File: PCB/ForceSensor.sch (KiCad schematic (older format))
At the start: 4 parts

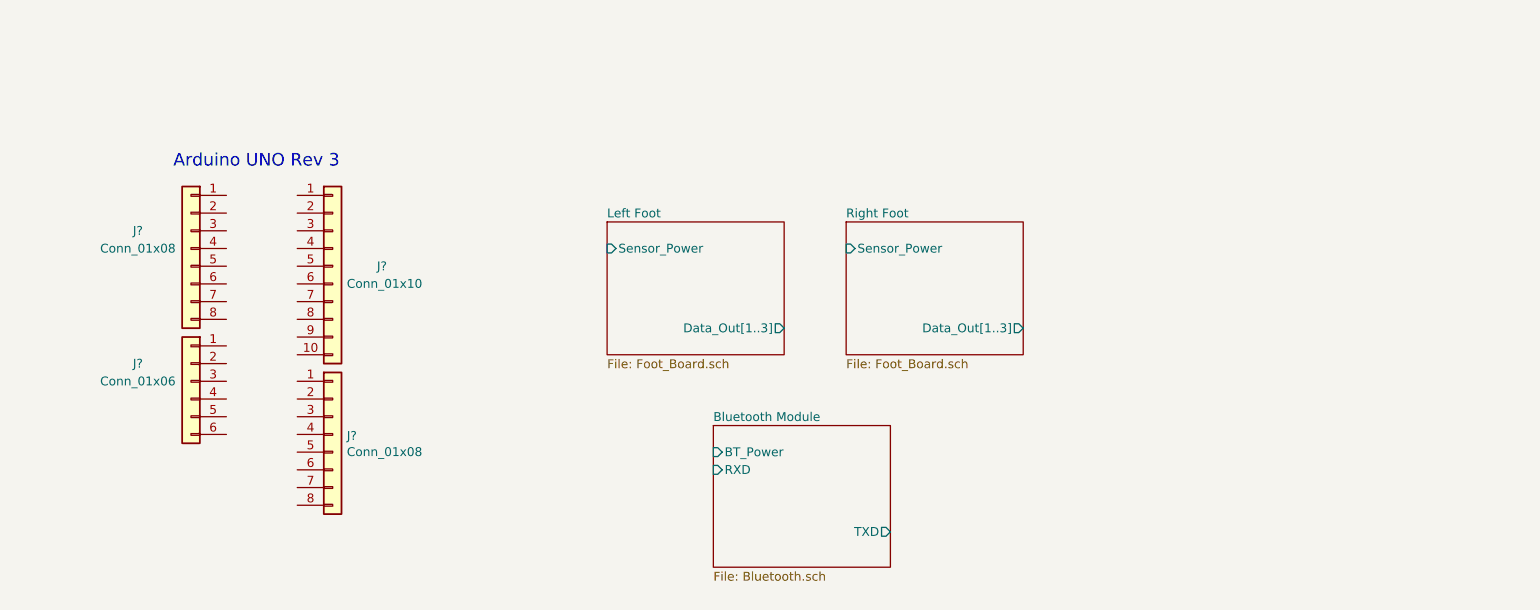
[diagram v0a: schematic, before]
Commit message: Finished schematic
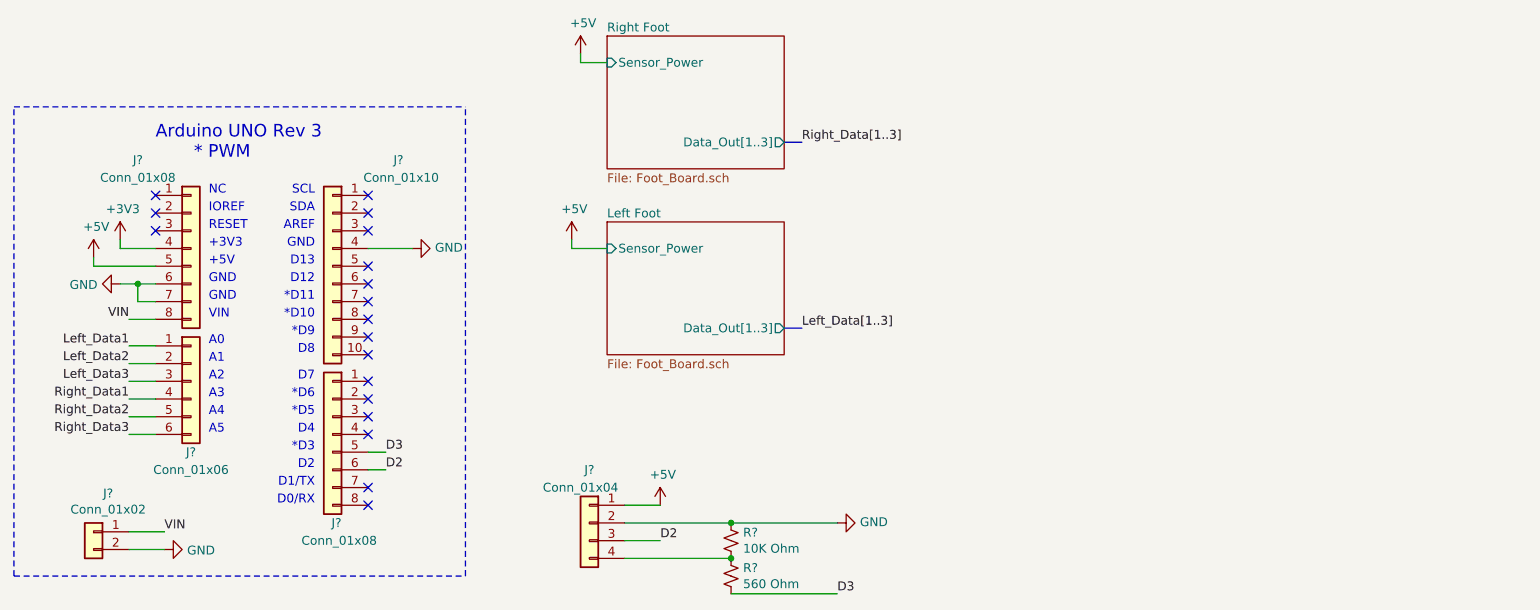
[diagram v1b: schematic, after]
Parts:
- added J?: Conn_01x04, symbol Connector_Generic:Conn_01x04
- added J?: Conn_01x02, symbol Connector_Generic:Conn_01x02
- added R?: 10K Ohm, symbol Device:R_Small_US
- added R?: 560 Ohm, symbol Device:R_Small_US
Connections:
- net GND: now reaches J?.4 (Pin_4)
- net GND: now also J?.6 (Pin_6), J?.7 (Pin_7), J?.2 (Pin_2), J?.2 (Pin_2), R?.1
- net D3: now reaches J?.5 (Pin_5)
- net D3: now also R?.2
- net D2: now reaches J?.6 (Pin_6)
- net D2: now also J?.3 (Pin_3)
- net +3V3: now reaches J?.4 (Pin_4)
- net +5V: now reaches J?.5 (Pin_5)
- net +5V: now also J?.1 (Pin_1)
- net VIN: now reaches J?.8 (Pin_8)
- net VIN: now also J?.1 (Pin_1)
- net Left_Data1: now reaches J?.1 (Pin_1)
- net Left_Data2: now reaches J?.2 (Pin_2)
- net Left_Data3: now reaches J?.3 (Pin_3)
- net Right_Data1: now reaches J?.4 (Pin_4)
- net Right_Data2: now reaches J?.5 (Pin_5)
- net Right_Data3: now reaches J?.6 (Pin_6)
- new net: J?.4 (Pin_4), R?.1, R?.2
- no-connect marks 0 -> 18
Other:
- note added: "*D10"
- note added: "*D11"
- note added: "*D3"
- note added: "*D5"
- note added: "*D6"
- note added: "*D9"
- note added: "+3V3"
- note added: "+5V"
- note added: "A0"
- note added: "A1"
- note added: "A2"
- note added: "A3"
- note added: "A4"
- note added: "A5"
- note added: "AREF"
- note added: "Arduino UNO Rev 3\n * PWM"
- note added: "D0/RX"
- note added: "D1/TX"
- note added: "D12"
- note added: "D13"
- note added: "D2"
- note added: "D4"
- note added: "D7"
- note added: "D8"
- note added: "GND"
- note added: "IOREF"
- note added: "NC"
- note added: "RESET"
- note added: "SCL"
- note added: "SDA"
- note added: "VIN"
- note removed: "Arduino UNO Rev 3"
- moved on the sheet: J?

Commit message: Small changes to schematic
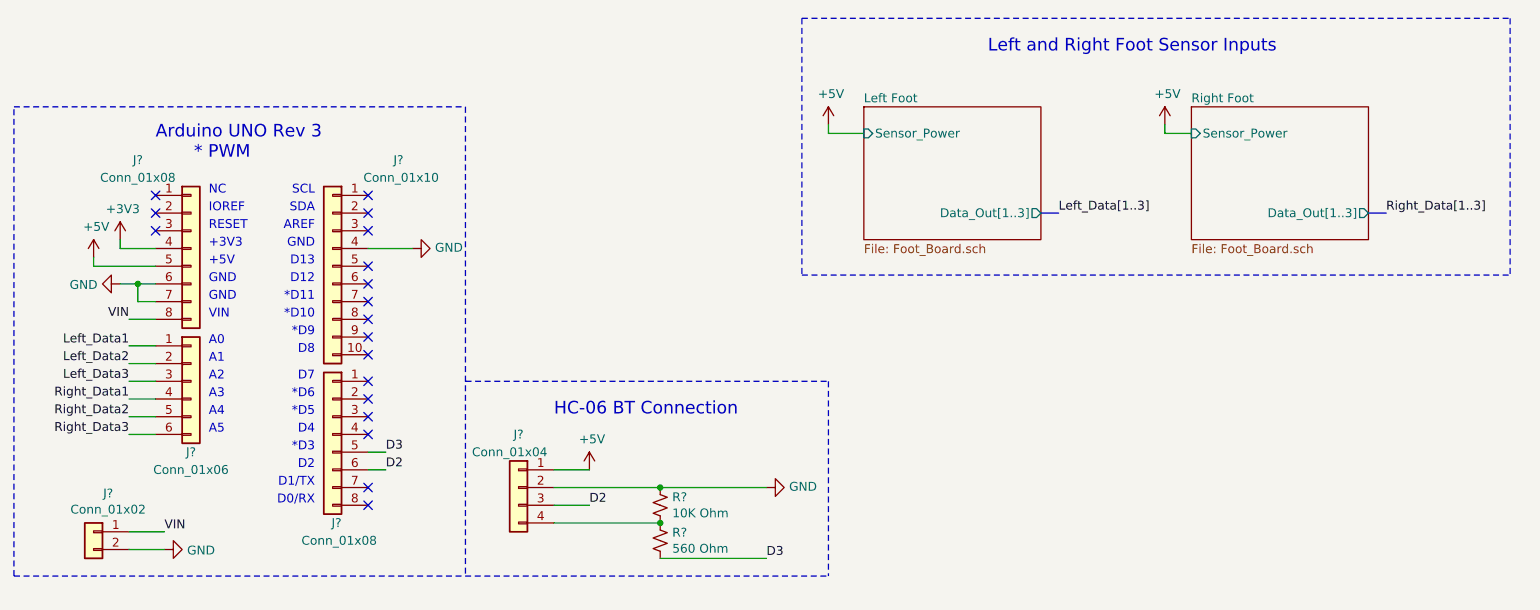
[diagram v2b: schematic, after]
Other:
- note added: "HC-06 BT Connection"
- note added: "Left and Right Foot Sensor Inputs"
- moved on the sheet: J?, R?
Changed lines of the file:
@@
 Arduino UNO Rev 3\n       * PWM
 $Sheet
-S 5400 2850 1000 750
+S 6850 2200 1000 750
 U 611C8367
 F0 "Left Foot" 50
 F1 "Foot_Board.sch" 50
-F2 "Sensor_Power" I L 5400 3000 50
-F3 "Data_Out[1..3]" O R 6400 3450 50
+F2 "Sensor_Power" I L 6850 2350 50
+F3 "Data_Out[1..3]" O R 7850 2800 50
 $EndSheet
 $Sheet
-S 5400 1800 1000 750
+S 8700 2200 1000 750
 U 611CB06B
 F0 "Right Foot" 50
 F1 "Foot_Board.sch" 50
-F2 "Sensor_Power" I L 5400 1950 50
-F3 "Data_Out[1..3]" O R 6400 2400 50
+F2 "Sensor_Power" I L 8700 2350 50
+F3 "Data_Out[1..3]" O R 9700 2800 50
 $EndSheet
 $Comp
@@
 L Connector_Generic:Conn_01x04 J?
 U 1 1 611DBB38
-P 5300 4550
+P 4900 4350
 AR Path="/611E7D97/611DBB38" Ref="J?"  Part="1"
 AR Path="/611DBB38" Ref="J?"  Part="1"
-F 0 "J?" H 5300 4850 50  0000 C CNN
-F 1 "Conn_01x04" H 5350 4750 50  0000 C CNN
-F 2 "" H 5300 4550 50  0001 C CNN
-F 3 "~" H 5300 4550 50  0001 C CNN
-	1    5300 4550
+F 0 "J?" H 4900 4650 50  0000 C CNN
+F 1 "Conn_01x04" H 4950 4550 50  0000 C CNN
+F 2 "" H 4900 4350 50  0001 C CNN
+F 3 "~" H 4900 4350 50  0001 C CNN
+	1    4900 4350
 	-1   0    0    -1
 $EndComp
@@
 L BPSDisplay:GND #PWR?
 U 1 1 611DBB3F
-P 6700 4550
+P 6300 4350
 AR Path="/611E7D97/611DBB3F" Ref="#PWR?"  Part="1"
 AR Path="/611DBB3F" Ref="#PWR?"  Part="1"
-F 0 "#PWR?" H 6700 4300 50  0001 C CNN
-F 1 "GND" V 6705 4422 50  0000 R CNN
-F 2 "" H 6700 4550 50  0000 C CNN
-F 3 "" H 6700 4550 50  0000 C CNN
-	1    6700 4550
+F 0 "#PWR?" H 6300 4100 50  0001 C CNN
+F 1 "GND" V 6305 4222 50  0000 R CNN
+F 2 "" H 6300 4350 50  0000 C CNN
+F 3 "" H 6300 4350 50  0000 C CNN
+	1    6300 4350
 	0    -1   -1   0
 $EndComp
@@
 L Device:R_Small_US R?
 U 1 1 611DBB45
-P 6100 4650
+P 5700 4450
 AR Path="/611E7D97/611DBB45" Ref="R?"  Part="1"
 AR Path="/611DBB45" Ref="R?"  Part="1"
-F 0 "R?" H 6168 4696 50  0000 L CNN
-F 1 "10K Ohm" H 6168 4605 50  0000 L CNN
-F 2 "" H 6100 4650 50  0001 C CNN
-F 3 "~" H 6100 4650 50  0001 C CNN
-	1    6100 4650
+F 0 "R?" H 5768 4496 50  0000 L CNN
+F 1 "10K Ohm" H 5768 4405 50  0000 L CNN
+F 2 "" H 5700 4450 50  0001 C CNN
+F 3 "~" H 5700 4450 50  0001 C CNN
+	1    5700 4450
 	1    0    0    -1
 $EndComp
@@
 L Device:R_Small_US R?
 U 1 1 611DBB4B
-P 6100 4850
+P 5700 4650
 AR Path="/611E7D97/611DBB4B" Ref="R?"  Part="1"
 AR Path="/611DBB4B" Ref="R?"  Part="1"
-F 0 "R?" H 6168 4896 50  0000 L CNN
-F 1 "560 Ohm" H 6168 4805 50  0000 L CNN
-F 2 "" H 6100 4850 50  0001 C CNN
-F 3 "~" H 6100 4850 50  0001 C CNN
-	1    6100 4850
-	1    0    0    -1
-$EndComp
-Wire Wire Line
-	5500 4650 5700 4650
-Wire Wire Line
-	5500 4550 6100 4550
-Wire Wire Line
-	5500 4750 6100 4750
-Wire Wire Line
-	6700 4550 6100 4550
-Connection ~ 6100 4550
-Connection ~ 6100 4750
-Wire Wire Line
-	6100 4950 6700 4950
-Wire Wire Line
-	5700 4450 5500 4450
-Wire Notes Line
-	4600 4850 4600 2200
+F 0 "R?" H 5768 4696 50  0000 L CNN
+F 1 "560 Ohm" H 5768 4605 50  0000 L CNN
+F 2 "" H 5700 4650 50  0001 C CNN
+F 3 "~" H 5700 4650 50  0001 C CNN
+	1    5700 4650
+	1    0    0    -1
+$EndComp
+Wire Wire Line
+	5100 4450 5300 4450
+Wire Wire Line
+	5100 4350 5700 4350
+Wire Wire Line
+	5100 4550 5700 4550
+Wire Wire Line
+	6300 4350 5700 4350
+Connection ~ 5700 4350
+Connection ~ 5700 4550
+Wire Wire Line
+	5700 4750 6300 4750
+Wire Wire Line
+	5300 4250 5100 4250
 $Comp
 L power:+3V3 #PWR?
@@
 L power:+5V #PWR?
 U 1 1 611ED85A
-P 5700 4450
-F 0 "#PWR?" H 5700 4300 50  0001 C CNN
-F 1 "+5V" H 5715 4623 50  0000 C CNN
-F 2 "" H 5700 4450 50  0001 C CNN
-F 3 "" H 5700 4450 50  0001 C CNN
-	1    5700 4450
-	1    0    0    -1
-$EndComp
-Text Label 6700 4950 0    50   ~ 0
+P 5300 4250
+F 0 "#PWR?" H 5300 4100 50  0001 C CNN
+F 1 "+5V" H 5315 4423 50  0000 C CNN
+F 2 "" H 5300 4250 50  0001 C CNN
+F 3 "" H 5300 4250 50  0001 C CNN
+	1    5300 4250
+	1    0    0    -1
+$EndComp
+Text Label 6300 4750 0    50   ~ 0
 D3
-Text Label 5700 4650 0    50   ~ 0
+Text Label 5300 4450 0    50   ~ 0
 D2
 $Comp
@@
 L power:+5V #PWR?
 U 1 1 611F02A4
-P 5200 2950
-F 0 "#PWR?" H 5200 2800 50  0001 C CNN
-F 1 "+5V" H 5215 3123 50  0000 C CNN
-F 2 "" H 5200 2950 50  0001 C CNN
-F 3 "" H 5200 2950 50  0001 C CNN
-	1    5200 2950
+P 6650 2300
+F 0 "#PWR?" H 6650 2150 50  0001 C CNN
+F 1 "+5V" H 6665 2473 50  0000 C CNN
+F 2 "" H 6650 2300 50  0001 C CNN
+F 3 "" H 6650 2300 50  0001 C CNN
+	1    6650 2300
 	1    0    0    -1
 $EndComp
@@
 L power:+5V #PWR?
 U 1 1 611F08C5
-P 5250 1900
-F 0 "#PWR?" H 5250 1750 50  0001 C CNN
-F 1 "+5V" H 5265 2073 50  0000 C CNN
-F 2 "" H 5250 1900 50  0001 C CNN
-F 3 "" H 5250 1900 50  0001 C CNN
-	1    5250 1900
-	1    0    0    -1
-$EndComp
-Wire Wire Line
-	5200 2950 5200 3000
-Wire Wire Line
-	5200 3000 5400 3000
-Wire Wire Line
-	5250 1900 5250 1950
-Wire Wire Line
-	5250 1950 5400 1950
+P 8550 2300
+F 0 "#PWR?" H 8550 2150 50  0001 C CNN
+F 1 "+5V" H 8565 2473 50  0000 C CNN
+F 2 "" H 8550 2300 50  0001 C CNN
+F 3 "" H 8550 2300 50  0001 C CNN
+	1    8550 2300
+	1    0    0    -1
+$EndComp
+Wire Wire Line
+	6650 2300 6650 2350
+Wire Wire Line
+	6650 2350 6850 2350
+Wire Wire Line
+	8550 2300 8550 2350
+Wire Wire Line
+	8550 2350 8700 2350
 Wire Notes Line
 	2050 4850 2050 2200
-Wire Notes Line
-	2050 4850 4600 4850
 Wire Notes Line
 	2050 2200 4600 2200
 Wire Bus Line
-	6400 3450 6500 3450
+	7850 2800 7950 2800
 Wire Bus Line
-	6400 2400 6500 2400
-Text Label 6500 2400 0    50   ~ 0
+	9700 2800 9800 2800
+Text Label 9800 2800 0    50   ~ 0
 Right_Data[1..3]
-Text Label 6500 3450 0    50   ~ 0
+Text Label 7950 2800 0    50   ~ 0
 Left_Data[1..3]
 Text Label 2700 3550 2    50   ~ 0
@@
 Wire Wire Line
 	2850 3550 2700 3550
+Text Notes 5100 3950 0    71   ~ 0
+HC-06 BT Connection
+Wire Notes Line
+	4600 3750 6650 3750
+Wire Notes Line
+	6650 3750 6650 4850
+Wire Notes Line
+	4600 2200 4600 4850
+Wire Notes Line
+	2050 4850 6650 4850
+Wire Notes Line
+	6500 1700 10500 1700
+Wire Notes Line
+	6500 3150 10500 3150
+Text Notes 7550 1900 0    71   ~ 0
+Left and Right Foot Sensor Inputs
+Wire Notes Line
+	6500 1700 6500 3150
+Wire Notes Line
+	10500 1700 10500 3150
 $EndSCHEMATC
